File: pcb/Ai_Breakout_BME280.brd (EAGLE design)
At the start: 100 x 80 mm, 10 parts, among them J1 1X04, J2 1X04NOFIRST, U1 BME280

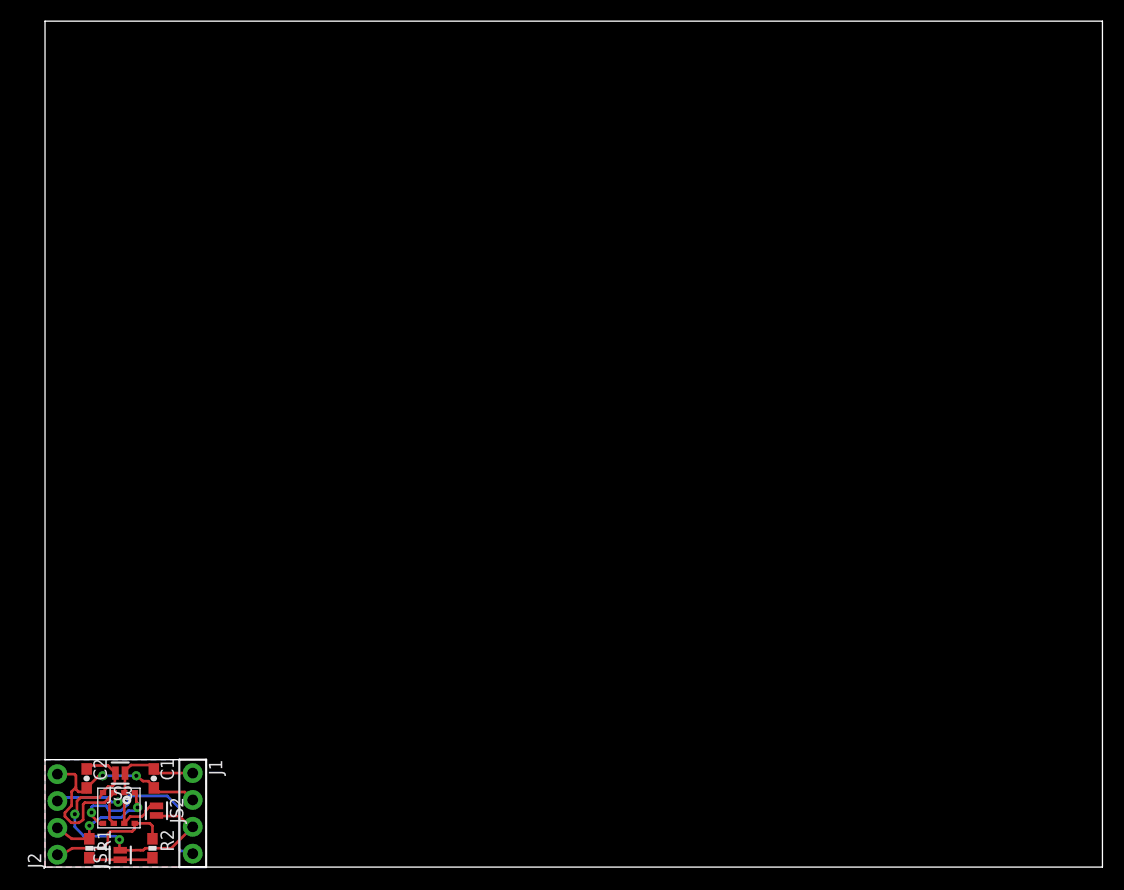
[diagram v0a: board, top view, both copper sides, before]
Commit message: first commit
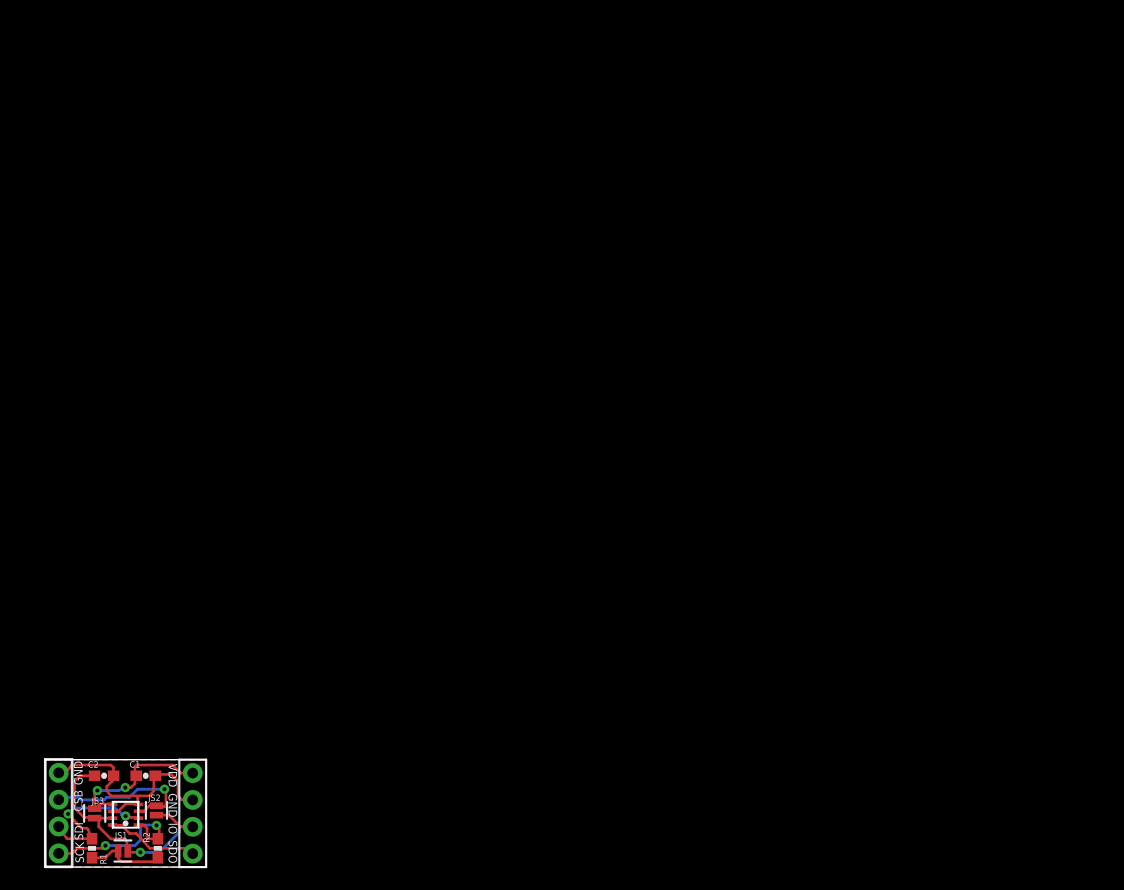
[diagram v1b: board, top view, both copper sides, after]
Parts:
- added U$2: AI-LOGOXS, Ai_Miscellany:AI-LOGO-XS
- moved JS3 4.51 mm to (4.70, 5.08), turned to 270 degrees
- moved C2 1.67 mm to (5.59, 8.64), turned to 0 degrees
- moved U1 0.90 mm to (7.62, 4.95), turned to 0 degrees
- moved C1 0.80 mm to (9.53, 8.64), turned to 0 degrees
- moved R2 0.51 mm to (10.7, 1.78)
- moved JS1 0.46 mm to (7.37, 1.52), turned to 0 degrees
- moved R1 0.25 mm to (4.45, 1.78)
- moved J2 0.18 mm to (1.30, 5.11)
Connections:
- net CSB: now also U1.2; no longer U1.6
- net GND: now also U1.1, U1.7; no longer U1.2, U1.5
- net SCK: now also U1.4; no longer U1.8
- net SDI: now also U1.3; no longer U1.7
- net SDO: now also U1.5; no longer U1.4
- net VDD: now also U1.8; no longer U1.1
- net VDDIO: now also U1.6; no longer U1.3
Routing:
- net SDO: track 17.6 -> 9.12 mm, vias 1 -> 0
- net GND: track 29.9 -> 24.0 mm, vias 2 -> 0
- net VDD: track 9.25 -> 15.1 mm, vias 0 -> 2
- net VDDIO: track 29.3 -> 25.6 mm, vias 2 -> 1
- net SCK: track 12.3 -> 15.4 mm, vias 0 -> 2
- net CSB: track 12.4 -> 15.5 mm
- net SDI: track 11.6 -> 14.6 mm
- net N$3: track 6.12 -> 7.47 mm
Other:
- board size 100 x 80 mm -> 15.2 x 10.2 mm
- board text added: "BME 280"
- board text added: "Breakout Board"
- board text added: "CSB"
- board text added: "GND"
- board text added: "IO"
- board text added: "SCK"
- board text added: "SDI"
- board text added: "SDO"
- board text added: "VDD"
- board text added: "www.acrobotic.com"
